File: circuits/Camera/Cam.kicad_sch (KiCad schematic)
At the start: 24 parts, among them J5 Conn_01x04_Male, J6 Conn_01x04_Male, J7 Conn_01x04_Male, J8 Conn_01x04_Male, Q12 S8550, Q13 SSM3J332R, Q14 S8550, Q15 S8550, Q16 SSM3J332R, Q17 S8550, Q18 S8550, Q19 SSM3J332R, Q20 S8550, Q7 S8550, Q8 SSM3J332R, Q9 S8550

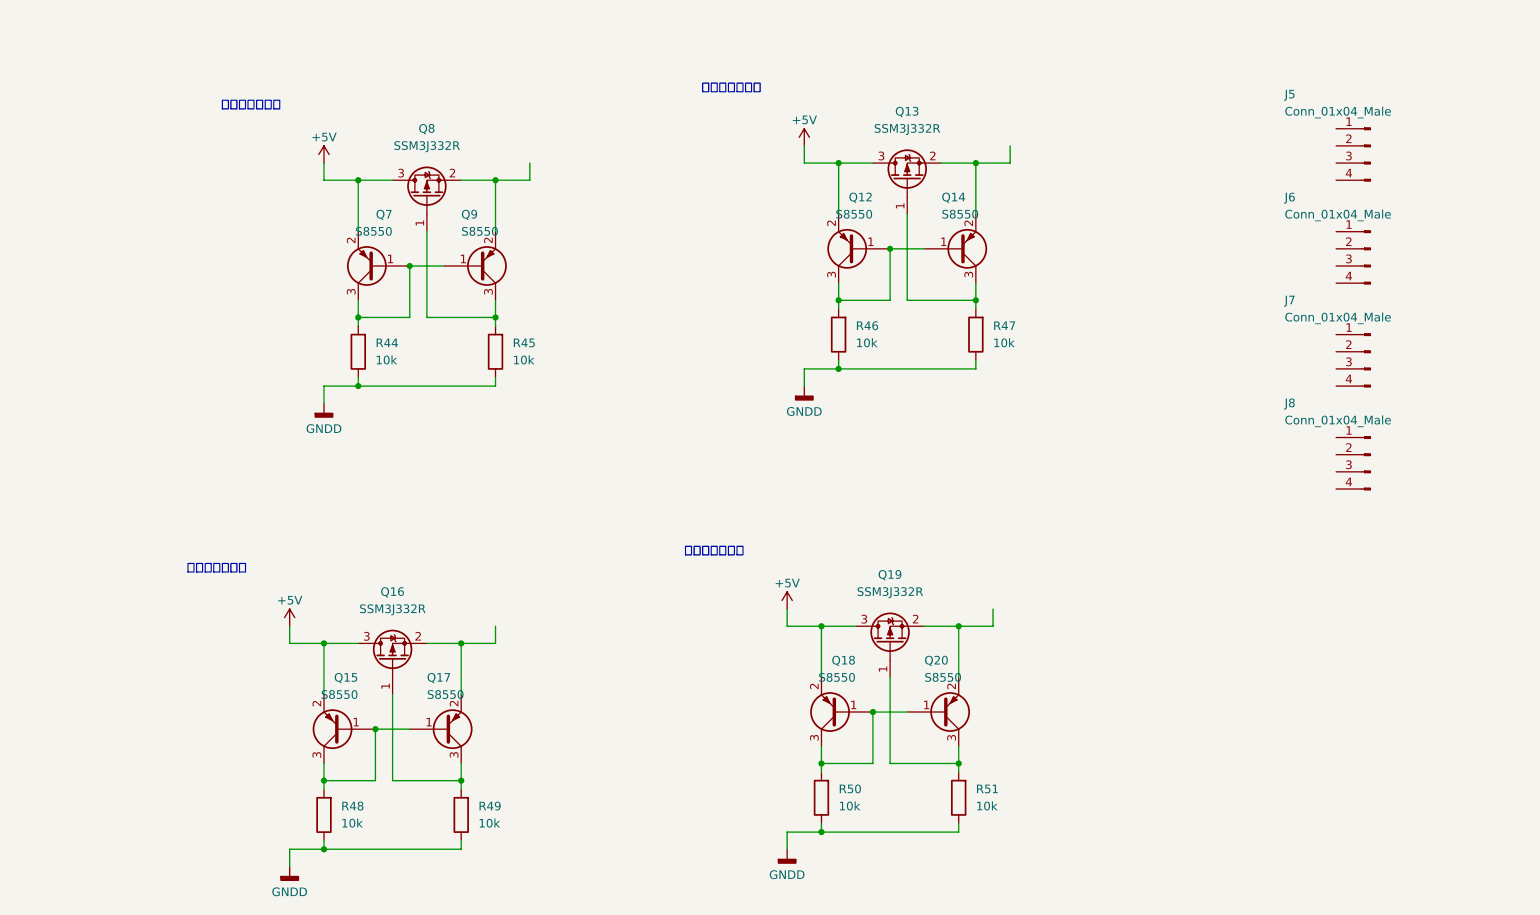
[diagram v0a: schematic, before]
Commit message: すてい
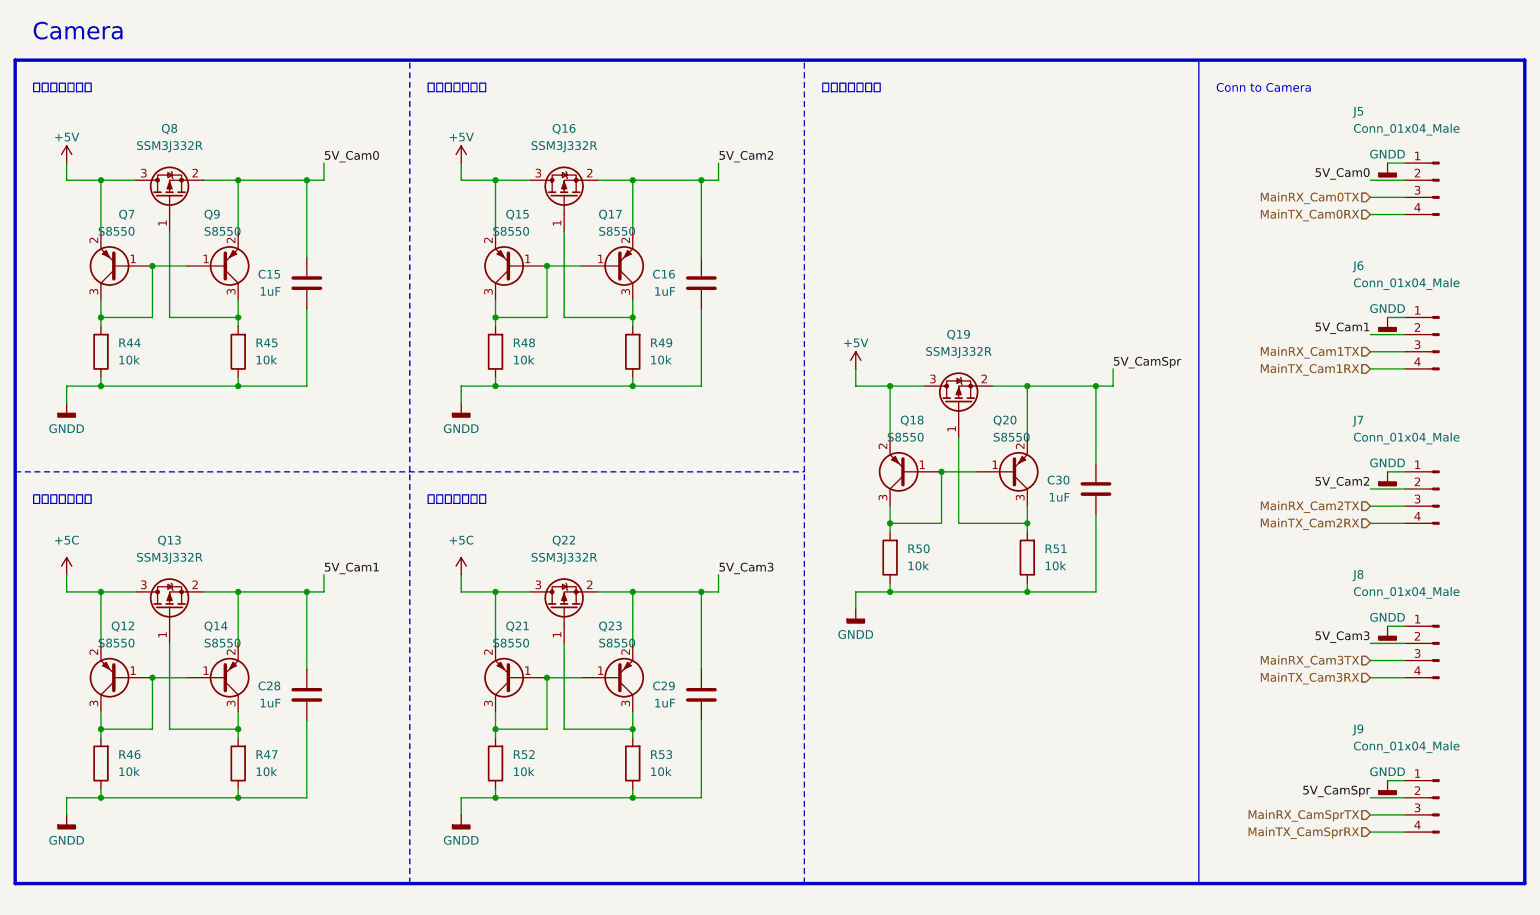
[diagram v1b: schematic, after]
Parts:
- added C15, C16, C28, C29, C30: 1uF, Capacitor_SMD:C_0402_1005Metric, symbol Device:C
- added J9: Conn_01x04_Male, Connector_Molex:Molex_SPOX_5267-04A_1x04_P2.50mm_Vertical, symbol Connector:Conn_01x04_Male
- added Q21, Q23: S8550, Package_TO_SOT_SMD:SOT-23, symbol Device:Q_PNP_BEC
- added Q22: SSM3J332R, Package_TO_SOT_SMD:SOT-23W, symbol Device:Q_PMOS_GSD
- added R52, R53: 10k, Resistor_SMD:R_0402_1005Metric, symbol Device:R
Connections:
- net +5V: no longer Q12.2 (E), Q13.3 (D)
- net GNDD: now also J5.1 (Pin_1), J6.1 (Pin_1), J7.1 (Pin_1), J8.1 (Pin_1), C15.2, C16.2, C28.2, C29.2, C30.2, J9.1 (Pin_1), R52.1, R53.1
- net 5V_Cam1: now reaches Q13.2 (S), Q14.2 (E)
- net 5V_Cam1: now also J6.2 (Pin_2), C28.1
- net 5V_Cam0: now reaches J5.2 (Pin_2)
- net 5V_Cam0: now also Q8.2 (S), Q9.2 (E), C15.1
- net MainRX_Cam0TX: now reaches J5.3 (Pin_3)
- net MainTX_Cam0RX: now reaches J5.4 (Pin_4)
- net 5V_Cam2: now reaches J7.2 (Pin_2)
- net 5V_Cam2: now also Q16.2 (S), Q17.2 (E), C16.1
- net MainRX_Cam2TX: now reaches J7.3 (Pin_3)
- net MainTX_Cam2RX: now reaches J7.4 (Pin_4)
- net 5V_Cam3: now reaches J8.2 (Pin_2)
- net 5V_Cam3: now also C29.1, Q22.2 (S), Q23.2 (E)
- net MainRX_Cam3TX: now reaches J8.3 (Pin_3)
- net MainTX_Cam3RX: now reaches J8.4 (Pin_4)
- net 5V_CamSpr: now reaches Q19.2 (S), Q20.2 (E)
- net 5V_CamSpr: now also C30.1, J9.2 (Pin_2)
- net MainRX_Cam1TX: now reaches J6.3 (Pin_3)
- net MainTX_Cam1RX: now reaches J6.4 (Pin_4)
- new net: Q21.1 (B), Q21.3 (C), Q23.1 (B), R52.2
- new net: Q22.1 (G), Q23.3 (C), R53.2
- new net +5C: Q12.2 (E), Q13.3 (D), Q21.2 (E), Q22.3 (D)
- new net MainRX_CamSprTX: J9.3 (Pin_3)
- new net MainTX_CamSprRX: J9.4 (Pin_4)
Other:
- note added: "Camera"
- note added: "Conn to Camera"
- moved on the sheet: J5, J6, J7, J8, Q12, Q13, Q14, Q15, Q16, Q17, Q18, Q19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
